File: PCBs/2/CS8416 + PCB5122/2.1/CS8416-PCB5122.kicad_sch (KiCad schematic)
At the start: 92 parts, among them J1 Conn_01x04_Pin, J10 Conn_01x02_Male, J11 Conn_01x02_Pin, J12 Conn_01x02_Pin, J13 Conn_01x02_Pin, J14 Conn_01x04_Pin, J15 Conn_01x02_Pin, J16 Conn_01x02_Pin, J17 Conn_01x02_Pin, J18 Conn_01x02_Pin, J19 Conn_01x02_Pin, J2 Conn_01x03_Pin, J20 Conn_01x02_Pin, J21 Conn_01x02_Male, J22 Conn_01x02_Male, J23 Conn_01x02_Pin, J24 Conn_01x02_Pin, J25 Conn_01x02_Pin, J3 Conn_01x02_Pin, J4 Conn_01x03_Pin, J5 Conn_01x02_Male, J6 CHANSEL, J7 Conn_01x02_Male, J8 Conn_01x02_Pin, J9 Conn_01x02_Pin, U1 ZLDO1117QG33TA, U2 PCM5142PWR, U3 CS8416-xZZ, X1 DFA-S3

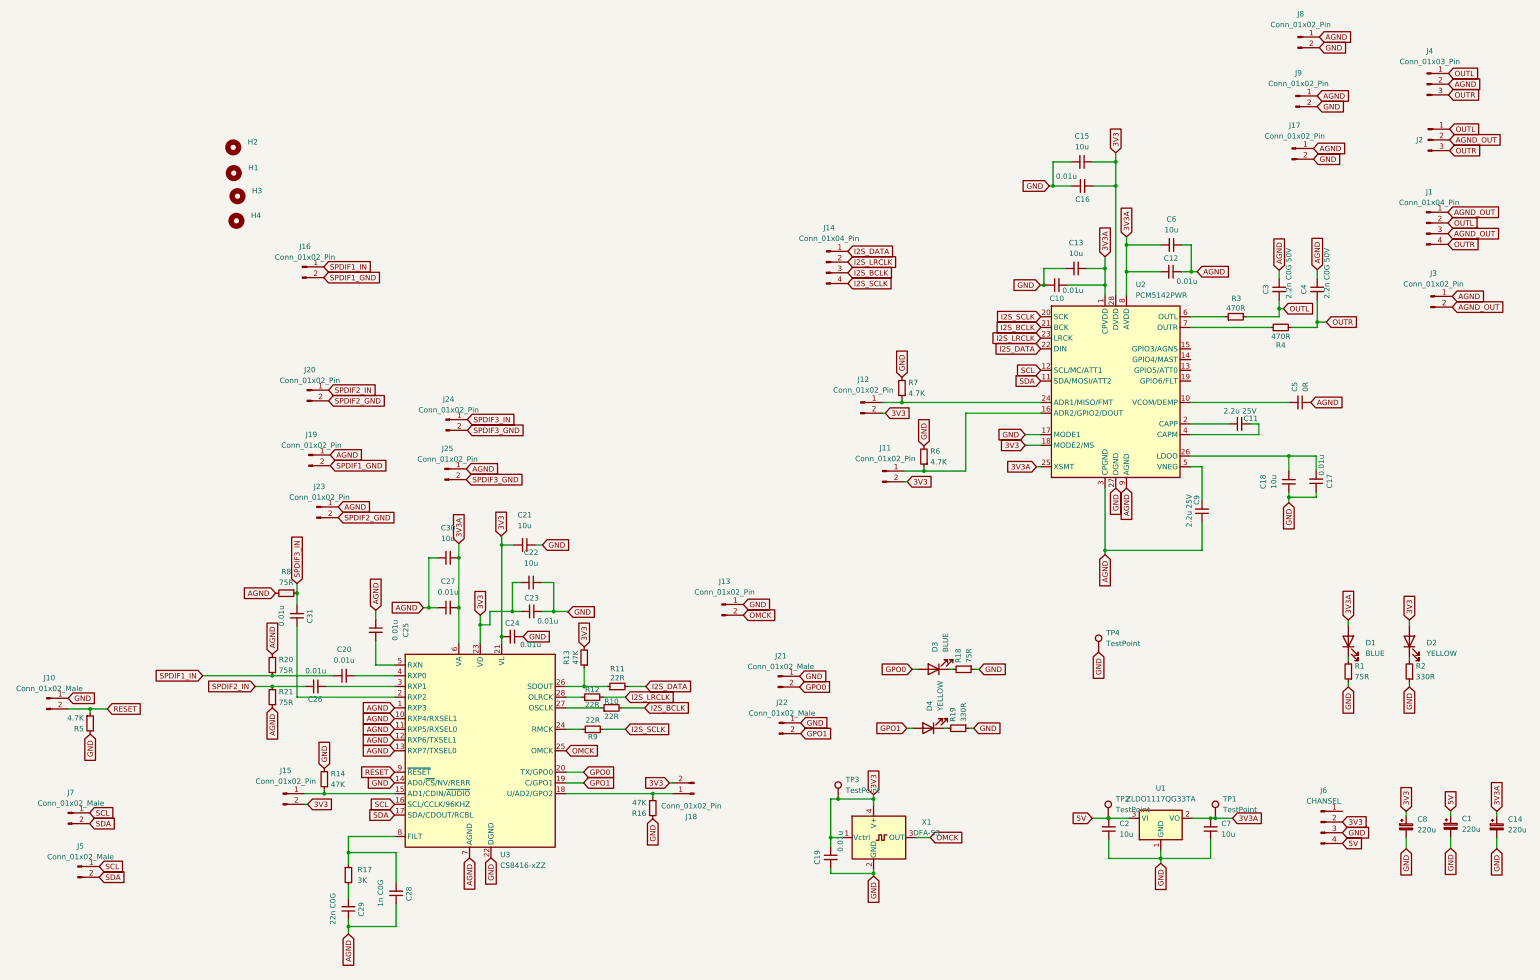
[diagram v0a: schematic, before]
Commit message: Updates
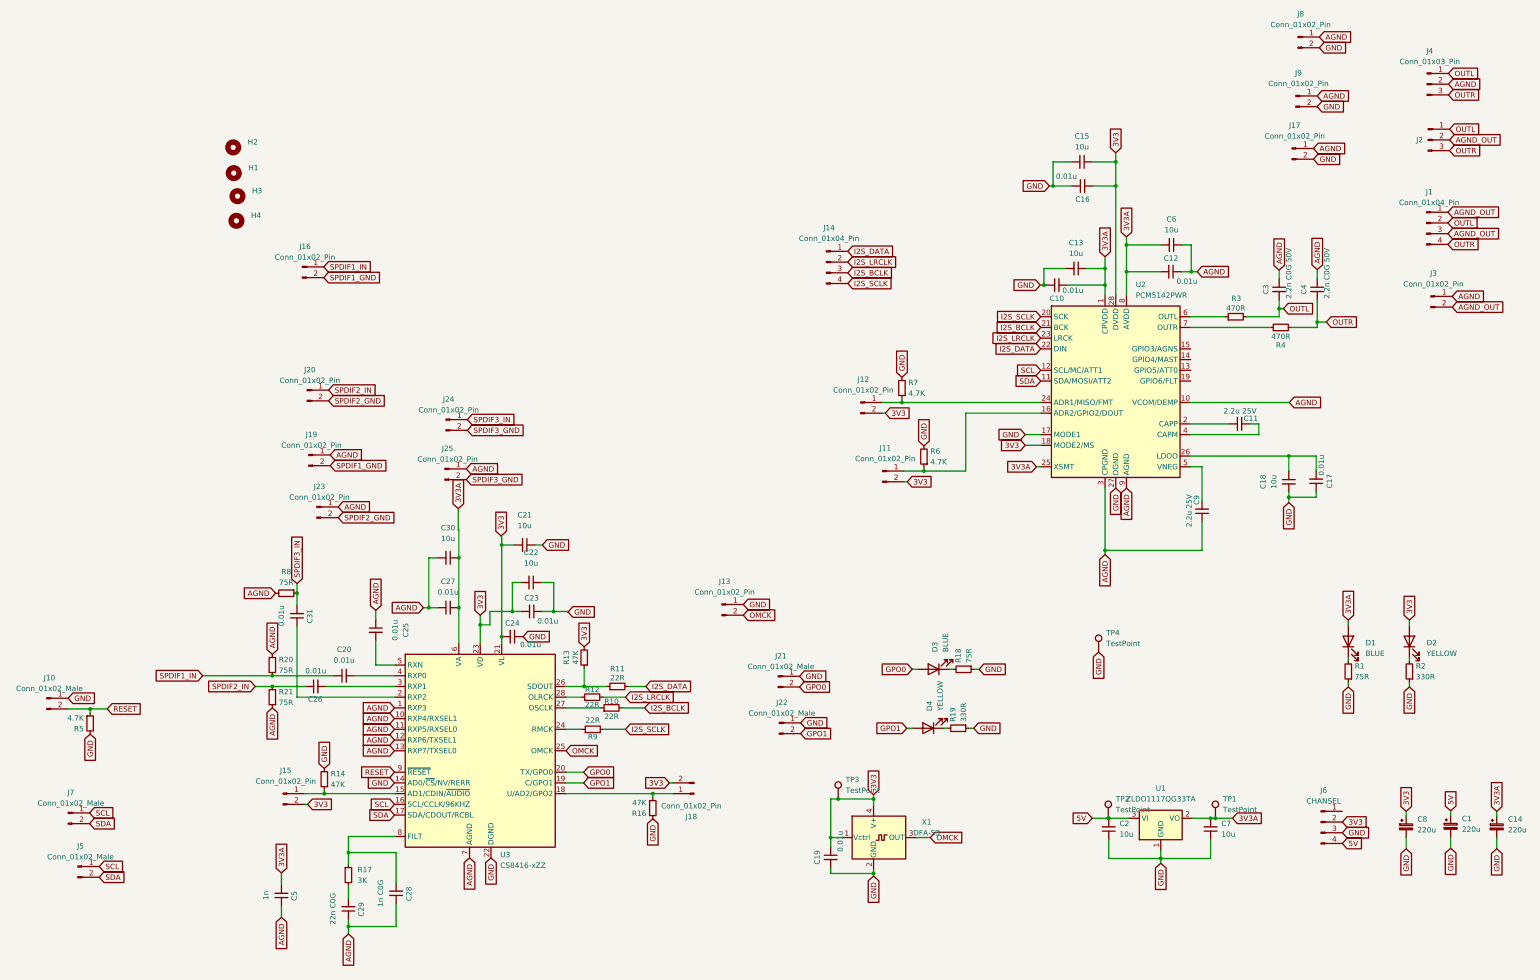
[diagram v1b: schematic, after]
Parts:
- C5: value 0R -> 1n; footprint Capacitor_SMD:C_1206_3216Metric_Pad1.33x1.80mm_HandSolder -> Capacitor_SMD:C_0805_2012Metric_Pad1.18x1.45mm_HandSolder
- R17: footprint Resistor_SMD:R_0603_1608Metric_Pad0.98x0.95mm_HandSolder -> Resistor_SMD:R_0805_2012Metric_Pad1.20x1.40mm_HandSolder
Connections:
- net 3V3A: now also C5.2
- net AGND: now also U2.10 (VCOM/DEMP)
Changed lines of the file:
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@@
     (stroke (width 0) (type default))
   )
+  (wire (pts (xy 128.651 147.828) (xy 128.778 147.828))
+    (stroke (width 0) (type default))
+  )
   (wire (pts (xy 216.916 220.726) (xy 219.456 220.726))
     (stroke (width 0) (type default))
@@
     (stroke (width 0) (type default))
   )
+  (wire (pts (xy 86.741 231.902) (xy 86.741 229.108))
+    (stroke (width 0) (type default))
+  )
   (wire (pts (xy 323.215 93.345) (xy 323.215 95.377))
     (stroke (width 0) (type default))
@@
     (stroke (width 0) (type default))
   )
-  (wire (pts (xy 128.778 151.003) (xy 128.778 154.432))
+  (wire (pts (xy 128.651 142.748) (xy 128.651 147.828))
     (stroke (width 0) (type default))
   )
@@
     (stroke (width 0) (type default))
   )
+  (wire (pts (xy 86.741 239.649) (xy 86.741 236.982))
+    (stroke (width 0) (type default))
+  )
   (wire (pts (xy 354.076 183.896) (xy 354.076 185.039))
     (stroke (width 0) (type default))
@@
     (stroke (width 0) (type default))
   )
+  (wire (pts (xy 128.778 147.828) (xy 128.778 154.432))
+    (stroke (width 0) (type default))
+  )
   (wire (pts (xy 163.83 184.912) (xy 158.496 184.912))
     (stroke (width 0) (type default))
@@
     )
   )
+  (global_label "AGND" (shape input) (at 86.741 239.649 270) (fields_autoplaced)
+    (effects (font (size 1.27 1.27)) (justify right))
+    (property "Intersheetrefs" "${INTERSHEET_REFS}" (at 86.741 247.5933 90)
+      (effects (font (size 1.27 1.27)) (justify right) hide)
+    )
+  )
   (global_label "GND" (shape input) (at 268.732 66.294 180) (fields_autoplaced)
     (effects (font (size 1.27 1.27)) (justify right))
@@
     )
   )
+  (global_label "3V3A" (shape input) (at 86.741 229.108 90) (fields_autoplaced)
+    (effects (font (size 1.27 1.27)) (justify left))
+    (property "Intersheetrefs" "${INTERSHEET_REFS}" (at 86.741 221.5266 90)
+      (effects (font (size 1.27 1.27)) (justify left) hide)
+    )
+  )
   (global_label "AGND" (shape input) (at 332.232 44.958 0) (fields_autoplaced)
     (effects (font (size 1.27 1.27)) (justify left))
@@
     )
   )
-  (global_label "3V3A" (shape input) (at 128.778 151.003 90) (fields_autoplaced)
+  (global_label "3V3A" (shape input) (at 128.651 142.748 90) (fields_autoplaced)
     (effects (font (size 1.27 1.27)) (justify left))
-    (property "Intersheetrefs" "${INTERSHEET_REFS}" (at 128.778 143.4216 90)
+    (property "Intersheetrefs" "${INTERSHEET_REFS}" (at 128.651 135.1666 90)
       (effects (font (size 1.27 1.27)) (justify left) hide)
     )
@@
     )
   )
-  (global_label "AGND" (shape input) (at 330.708 117.602 0) (fields_autoplaced)
+  (global_label "AGND" (shape input) (at 325.628 117.602 0) (fields_autoplaced)
     (effects (font (size 1.27 1.27)) (justify left))
-    (property "Intersheetrefs" "${INTERSHEET_REFS}" (at 338.6523 117.602 0)
+    (property "Intersheetrefs" "${INTERSHEET_REFS}" (at 333.5723 117.602 0)
       (effects (font (size 1.27 1.27)) (justify left) hide)
     )
@@
     )
   )
+  (symbol (lib_id "Device:C_Small") (at 86.741 234.442 180) (unit 1)
+    (in_bom yes) (on_board yes) (dnp no)
+    (property "Reference" "C5" (at 89.789 234.569 90)
+      (effects (font (size 1.27 1.27)))
+    )
+    (property "Value" "1n" (at 83.058 234.4357 90)
+      (effects (font (size 1.27 1.27)))
+    )
+    (property "Footprint" "Capacitor_SMD:C_0805_2012Metric_Pad1.18x1.45mm_HandSolder" (at 86.741 234.442 0)
+      (effects (font (size 1.27 1.27)) hide)
+    )
+    (property "Datasheet" "~" (at 86.741 234.442 0)
+      (effects (font (size 1.27 1.27)) hide)
+    )
+    (pin "1")
+    (pin "2")
+    (instances
+      (project "CS8416-PCB5122"
+        (path "/2ceb088e-6d49-4b44-ae2d-2365af779427"
+          (reference "C5") (unit 1)
+        )
+      )
+    )
+  )
   (symbol (lib_id "Connector:Conn_01x02_Pin") (at 359.156 92.456 0) (unit 1)
     (in_bom yes) (on_board yes) (dnp no) (fields_autoplaced)
@@
       (effects (font (size 1.27 1.27)) (justify left))
     )
-    (property "Footprint" "Resistor_SMD:R_0603_1608Metric_Pad0.98x0.95mm_HandSolder" (at 102.616 229.616 0)
+    (property "Footprint" "Resistor_SMD:R_0805_2012Metric_Pad1.20x1.40mm_HandSolder" (at 102.616 229.616 0)
       (effects (font (size 1.27 1.27)) hide)
     )
@@
         )
       )
-    )
-  )
-  (symbol (lib_id "Device:C_Small") (at 328.168 117.602 270) (unit 1)
-    (in_bom yes) (on_board yes) (dnp no) (fields_autoplaced)
-    (property "Reference" "C5" (at 326.8916 115.062 0)
-      (effects (font (size 1.27 1.27)) (justify right))
-    )
-    (property "Value" "0R" (at 329.4316 115.062 0)
-      (effects (font (size 1.27 1.27)) (justify right))
-    )
-    (property "Footprint" "Capacitor_SMD:C_1206_3216Metric_Pad1.33x1.80mm_HandSolder" (at 328.168 117.602 0)
-      (effects (font (size 1.27 1.27)) hide)
-    )
-    (property "Datasheet" "~" (at 328.168 117.602 0)
-      (effects (font (size 1.27 1.27)) hide)
-    )
-    (pin "1")
-    (pin "2")
-    (instances
-      (project "CS8416-PCB5122"
-        (path "/2ceb088e-6d49-4b44-ae2d-2365af779427"
-          (reference "C5") (unit 1)
-        )
-      )
